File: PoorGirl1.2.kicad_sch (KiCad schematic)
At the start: 34 parts, among them J1 NES_Connector-Connector, J2 Conn_01x06_Pin, U1 EPM570T100, U2 Memory_Flash_29GL01G, U3 K6F2008T2E, U4 FM1808B-SG, U5 AMS1117-3.3

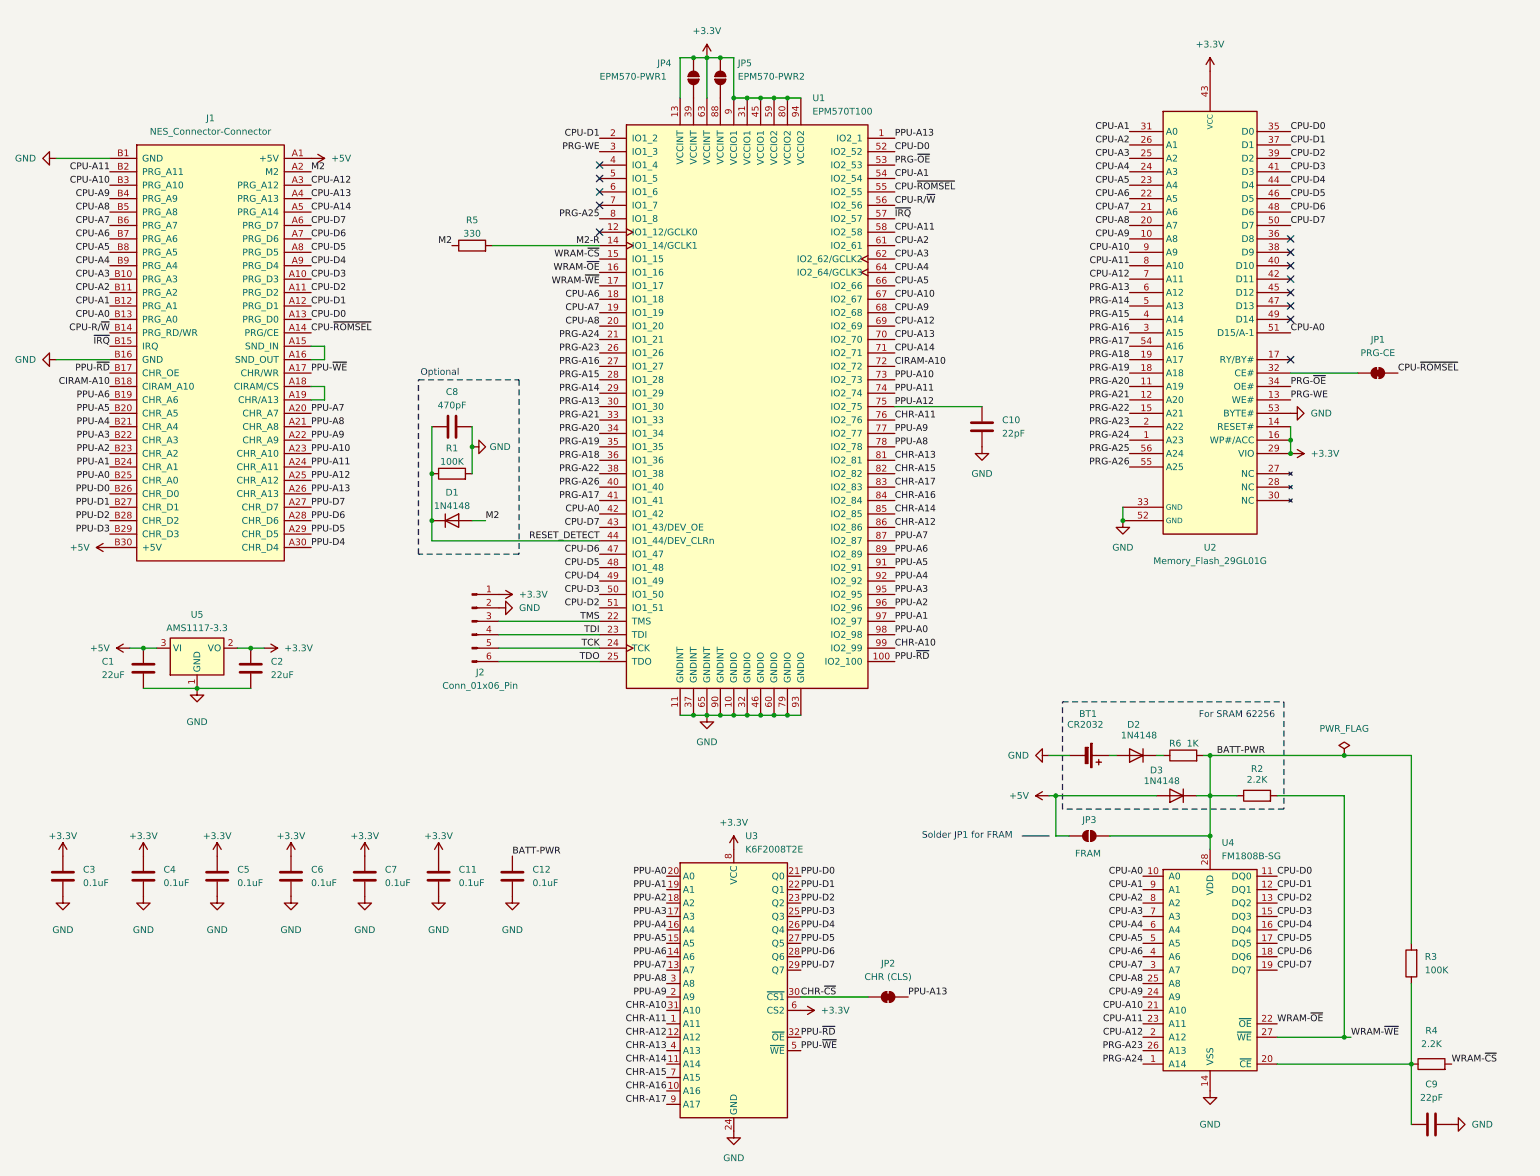
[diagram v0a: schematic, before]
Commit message: Mapper 69 fix
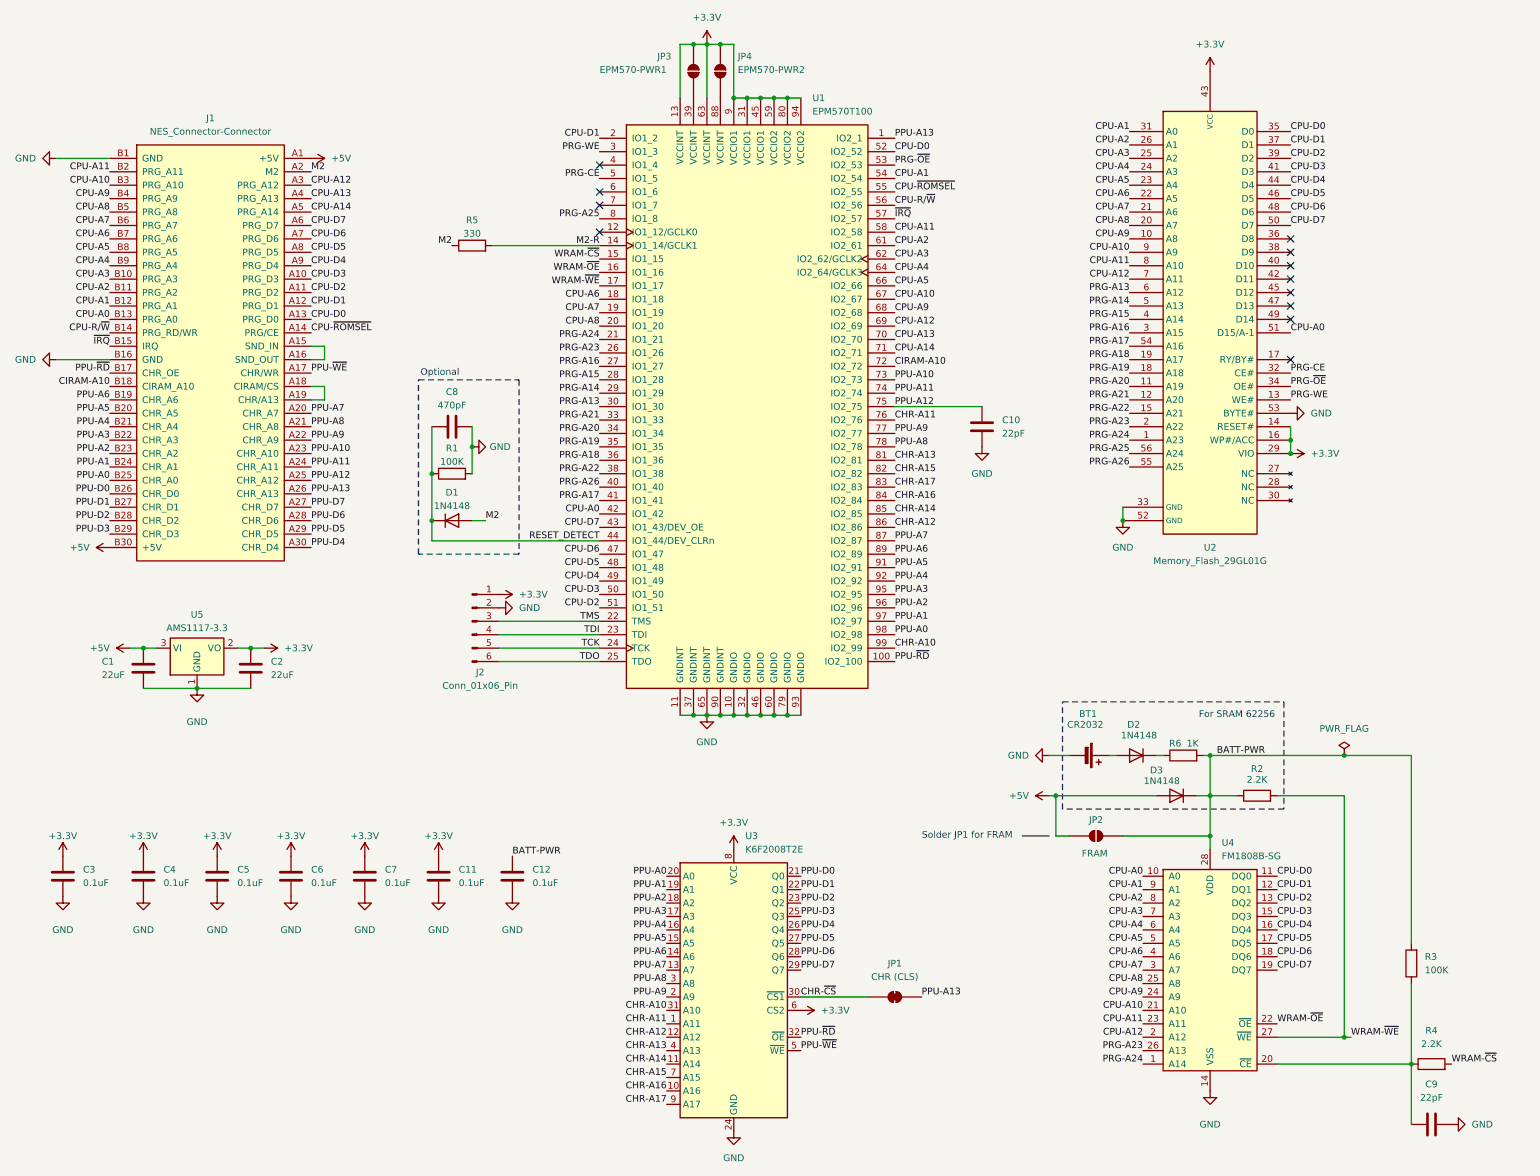
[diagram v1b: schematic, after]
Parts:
- removed JP1: PRG-CE, Jumper:SolderJumper-2_P1.3mm_Bridged_RoundedPad1.0x1.5mm, symbol Jumper:SolderJumper_2_Bridged
- renumbered JP2 to JP1, JP3 to JP2, JP4 to JP3, JP5 to JP4
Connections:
- net PRG-CE: now reaches U2.32 (CE#)
- net PRG-CE: now also U1.5 (IO1_5)
- no-connect marks 13 -> 12
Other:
- moved on the sheet: JP1, JP2, JP3, JP4
